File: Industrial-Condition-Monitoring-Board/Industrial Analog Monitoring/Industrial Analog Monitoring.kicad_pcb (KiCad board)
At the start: 2 copper layers, 60 parts, among them J1 +12V i/p, J2 Temperature Sensor Input, J3 LDR input, J4 Pressure input, Q1 BC547, Q2 BC547, Q3 BC547, Q4 BC547, U1 LM7805_TO220, U2 LM358, U3 LM339

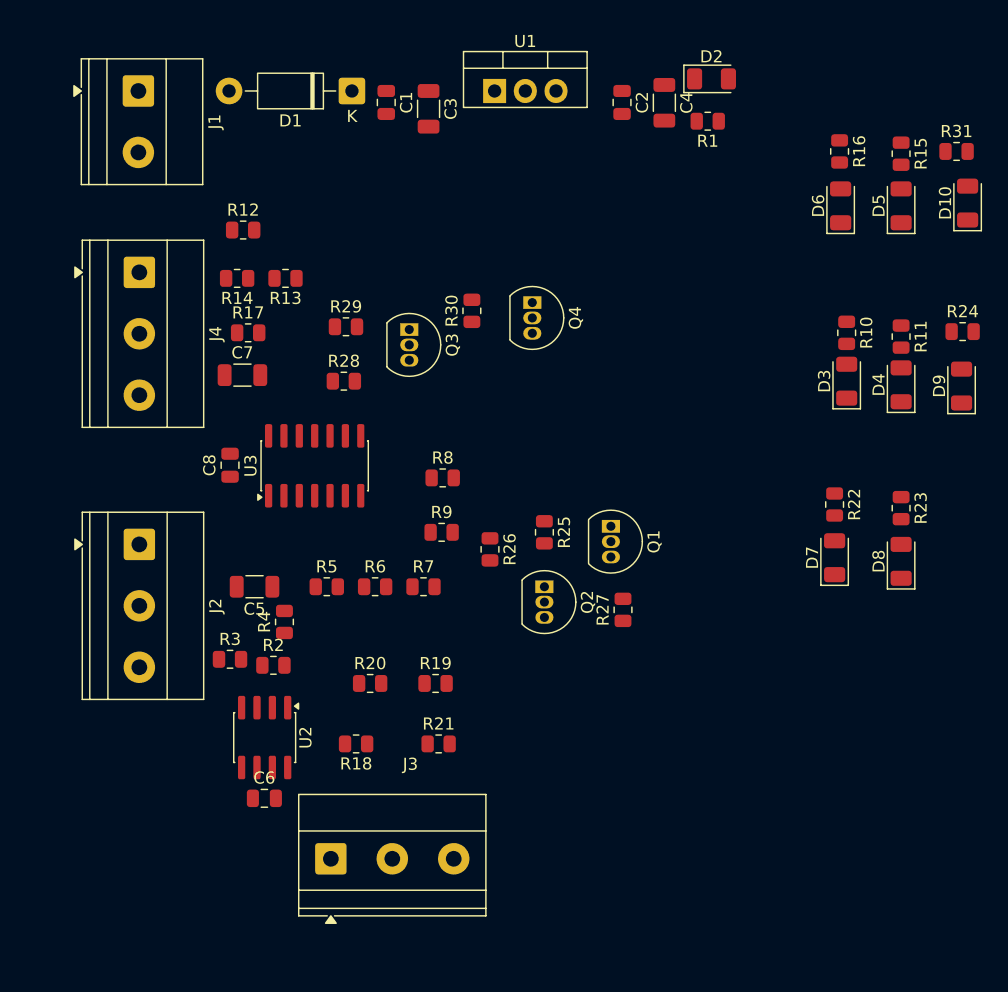
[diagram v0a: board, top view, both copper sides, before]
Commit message: Updates
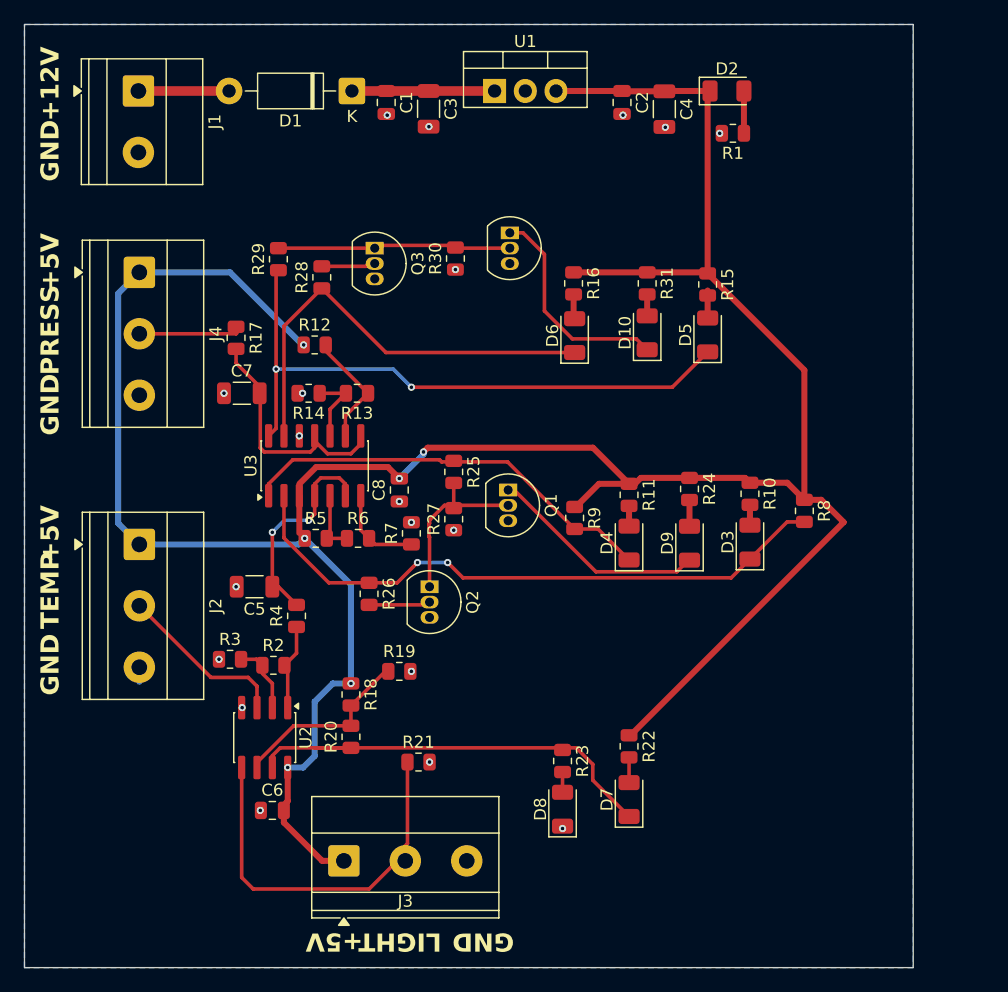
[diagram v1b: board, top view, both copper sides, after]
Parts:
- moved R23 34.9 mm to (61.0, 72.9)
- moved D8 34.7 mm to (61.0, 76.9)
- moved R8 30.0 mm to (81.0, 52.2), turned to -90 degrees
- moved D10 28.6 mm to (68.0, 37.5)
- moved R31 27.8 mm to (68.0, 33.4), turned to -90 degrees
- moved D7 26.2 mm to (66.5, 76.1)
- moved R22 26.2 mm to (66.5, 71.7)
- moved R24 26.1 mm to (71.5, 50.4), turned to -90 degrees
- moved D4 26.0 mm to (66.5, 54.9)
- moved R11 26.0 mm to (66.5, 50.9)
- moved D9 26.0 mm to (71.5, 54.9)
- moved R16 24.6 mm to (61.9, 33.4)
- moved D6 24.5 mm to (62.0, 37.7)
- moved R15 19.3 mm to (73.0, 33.5)
- moved D5 19.2 mm to (73.0, 37.7)
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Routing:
- net +5V: track 0.00 -> 235.2 mm, vias 0 -> 6
- net /PRES_GT_3.33_N: track 0.00 -> 51.6 mm, vias 0 -> 2
- net /TEMP_GT_60_N: track 0.00 -> 51.2 mm, vias 0 -> 2
- net /LIGHT_CONDITION: track 0.00 -> 36.9 mm
- net /PRES_GT_1.66_N: track 0.00 -> 36.6 mm
- net /TEMP_GT_40_N: track 0.00 -> 35.0 mm
- net Net-(J3-Pin_2): track 0.00 -> 31.8 mm
- net /PRESSURE-CONDITIONED: track 0.00 -> 20.4 mm
- net Net-(Q3-C): track 0.00 -> 19.3 mm
- net Net-(D9-K): track 0.00 -> 18.2 mm
- net Net-(D10-K): track 0.00 -> 18.1 mm
- net /TEMP_CONDITIONED: track 0.00 -> 17.7 mm, vias 0 -> 2
- net Net-(U2B--): track 0.00 -> 15.5 mm
- net Net-(Q1-B): track 0.00 -> 14.6 mm
- net /TEMP_INPUT: track 0.00 -> 14.3 mm
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- added copper zone on B.Cu, net GND
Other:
- board outline added: 73.5 x 78 mm
- board text added: "+12V"
- board text added: "+5V"
- board text added: "GND"
- board text added: "LIGHT"
- board text added: "PRESS"
- board text added: "TEMP"
